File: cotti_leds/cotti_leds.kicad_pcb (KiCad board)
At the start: 2 copper layers, 63.5 x 20.3 mm, 39 parts, among them J1 Pmod GPIO 1x06 pin, Q1 PMOS Kp=0.2A/V² |Vth|=0.8V, Q2 NMOS, Q3 PMOS Kp=0.2A/V² |Vth|=0.8V, Q4 NMOS, Q5 PMOS Kp=0.2A/V² |Vth|=0.8V, Q6 NMOS, Q7 PMOS Kp=0.2A/V² |Vth|=0.8V, Q8 NMOS, SW1 SW_4PDT

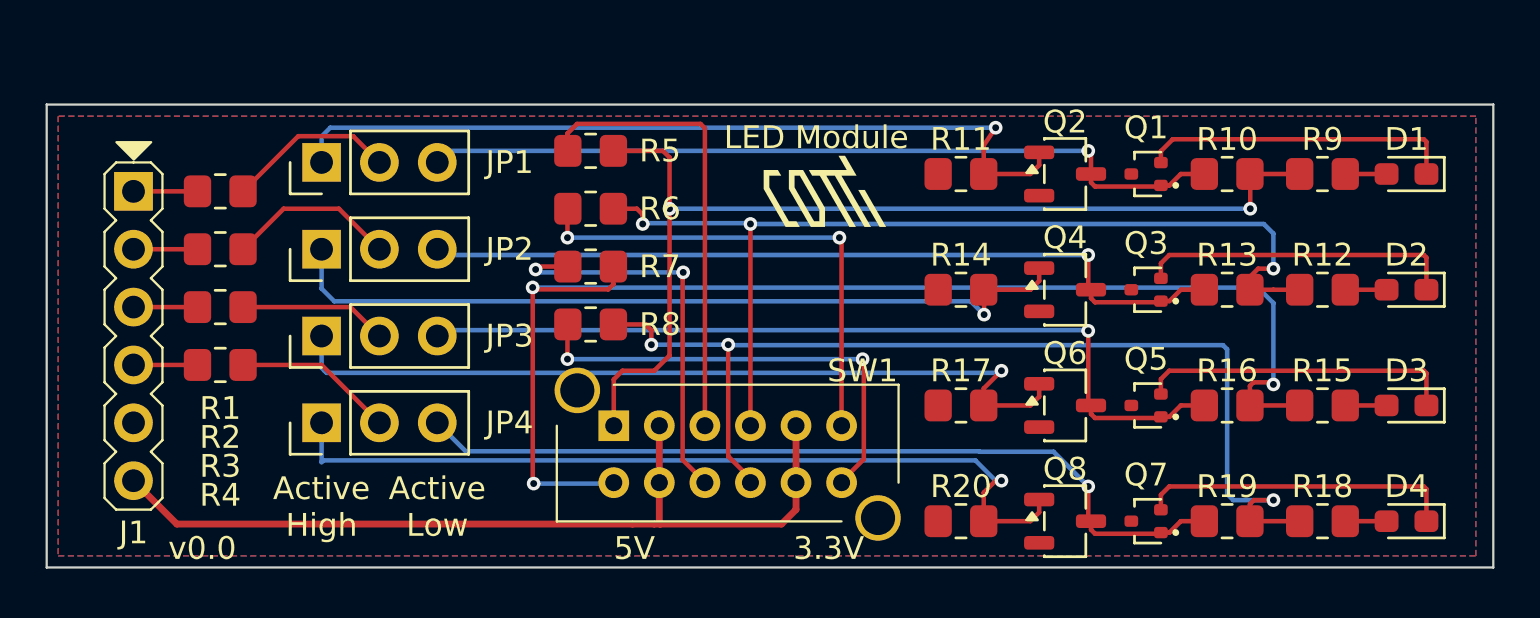
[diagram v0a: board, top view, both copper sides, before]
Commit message: feat: cotti_leds v0.0
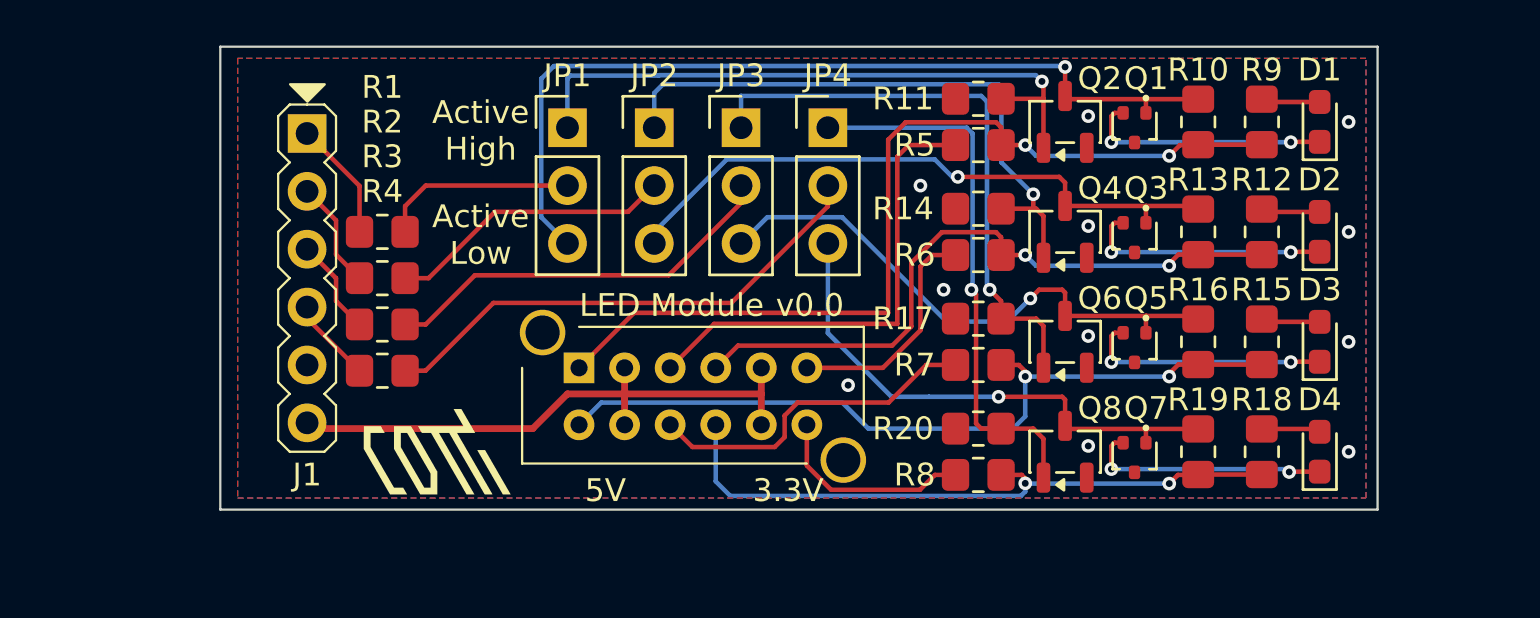
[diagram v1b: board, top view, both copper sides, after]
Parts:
- removed the REF** at (130.5, 101.9)
- added REF**: cotti_logo_filled H=3mm T=0.3mm, Cotti_logo:cotti_logo_filled H=3mm T=0.3mm, F.Cu at (113.0, 113.2)
- moved JP4 25.7 mm to (133.3, 100.1), turned to 0 degrees
- moved JP3 20.6 mm to (129.5, 100.1), turned to 0 degrees
- moved R8 18.3 mm to (140.0, 115.3)
- moved R7 17.6 mm to (140.0, 110.5)
- moved R6 17.1 mm to (140.0, 105.7)
- moved R5 17.0 mm to (140.0, 100.8)
- moved JP2 15.5 mm to (125.7, 100.1), turned to 0 degrees
- moved JP1 10.9 mm to (121.9, 100.1), turned to 0 degrees
- moved J1 8.03 mm to (110.5, 100.3)
- moved R1 7.33 mm to (113.8, 104.6)
- moved R2 7.22 mm to (113.8, 106.7)
- moved R3 7.15 mm to (113.8, 108.7)
- moved R4 7.12 mm to (113.8, 110.7)
- moved D4 4.88 mm to (154.9, 114.3), turned to 90 degrees
- moved D3 4.72 mm to (154.9, 109.5), turned to 90 degrees
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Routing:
- net /vcc3: track 57.2 -> 34.5 mm, vias 3 -> 2
- net /vcc4: track 46.8 -> 28.9 mm, vias 3 -> 2
- net /io4: track 7.04 -> 22.5 mm
- net /vcc2: track 44.0 -> 29.4 mm, vias 3 -> 2
- net /io4_L: track 37.0 -> 23.2 mm
- net /io4_H: track 37.4 -> 24.2 mm
- net /io3_L: track 37.7 -> 24.9 mm
- net VCC: track 38.1 -> 25.7 mm
- net Net-(R6-Pad1): track 21.5 -> 10.2 mm, vias 2 -> 0
- net Net-(R8-Pad1): track 20.3 -> 9.08 mm, vias 2 -> 0
- net /io3: track 6.51 -> 17.7 mm
- net /io3_H: track 36.4 -> 25.9 mm
- net /io2_H: track 35.5 -> 26.7 mm
- net /io1_H: track 36.2 -> 28.0 mm
- net /io2_L: track 35.9 -> 27.9 mm
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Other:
- board size 63.5 x 20.3 mm -> 50.8 x 20.3 mm
